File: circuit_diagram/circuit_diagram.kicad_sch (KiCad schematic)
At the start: 26 parts, among them J1 Sheild Power, M1 Stepper_Motor_bipolar, M2 Stepper_Motor_bipolar, M3 Stepper_Motor_bipolar, M4 Stepper_Motor_bipolar, M5 Motor_DC, SW1 SW_DPST_x2, SW2 SW_Push, U1 DEVKIT_V1_ESP32-WROOM-32

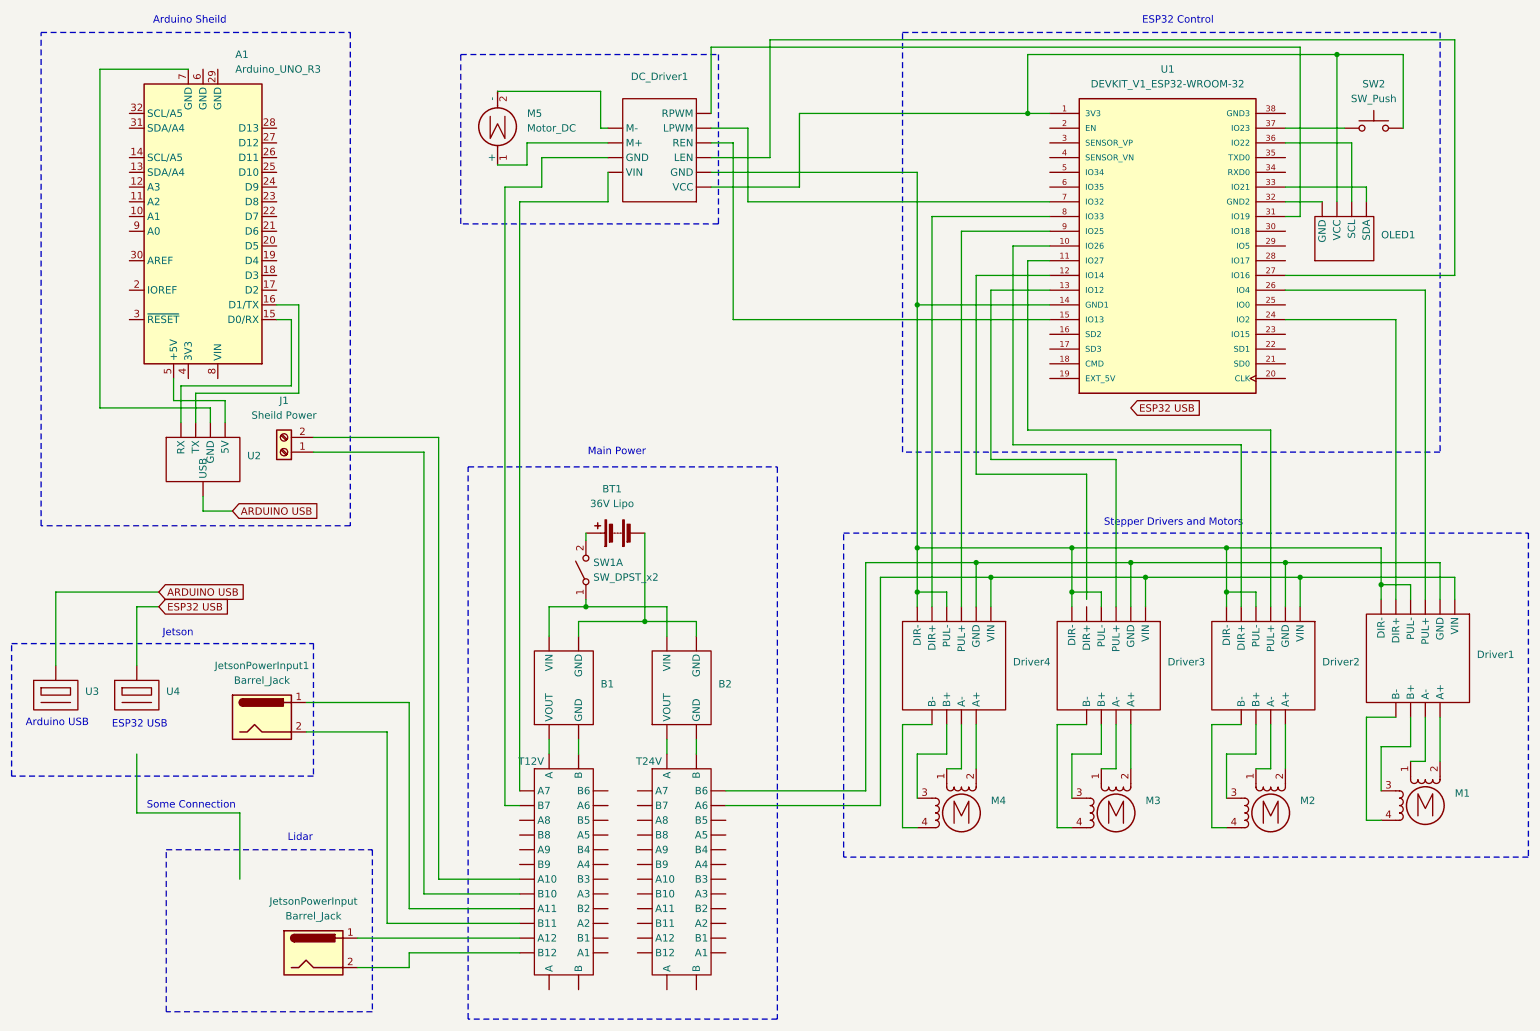
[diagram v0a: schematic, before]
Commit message: Drill Driver
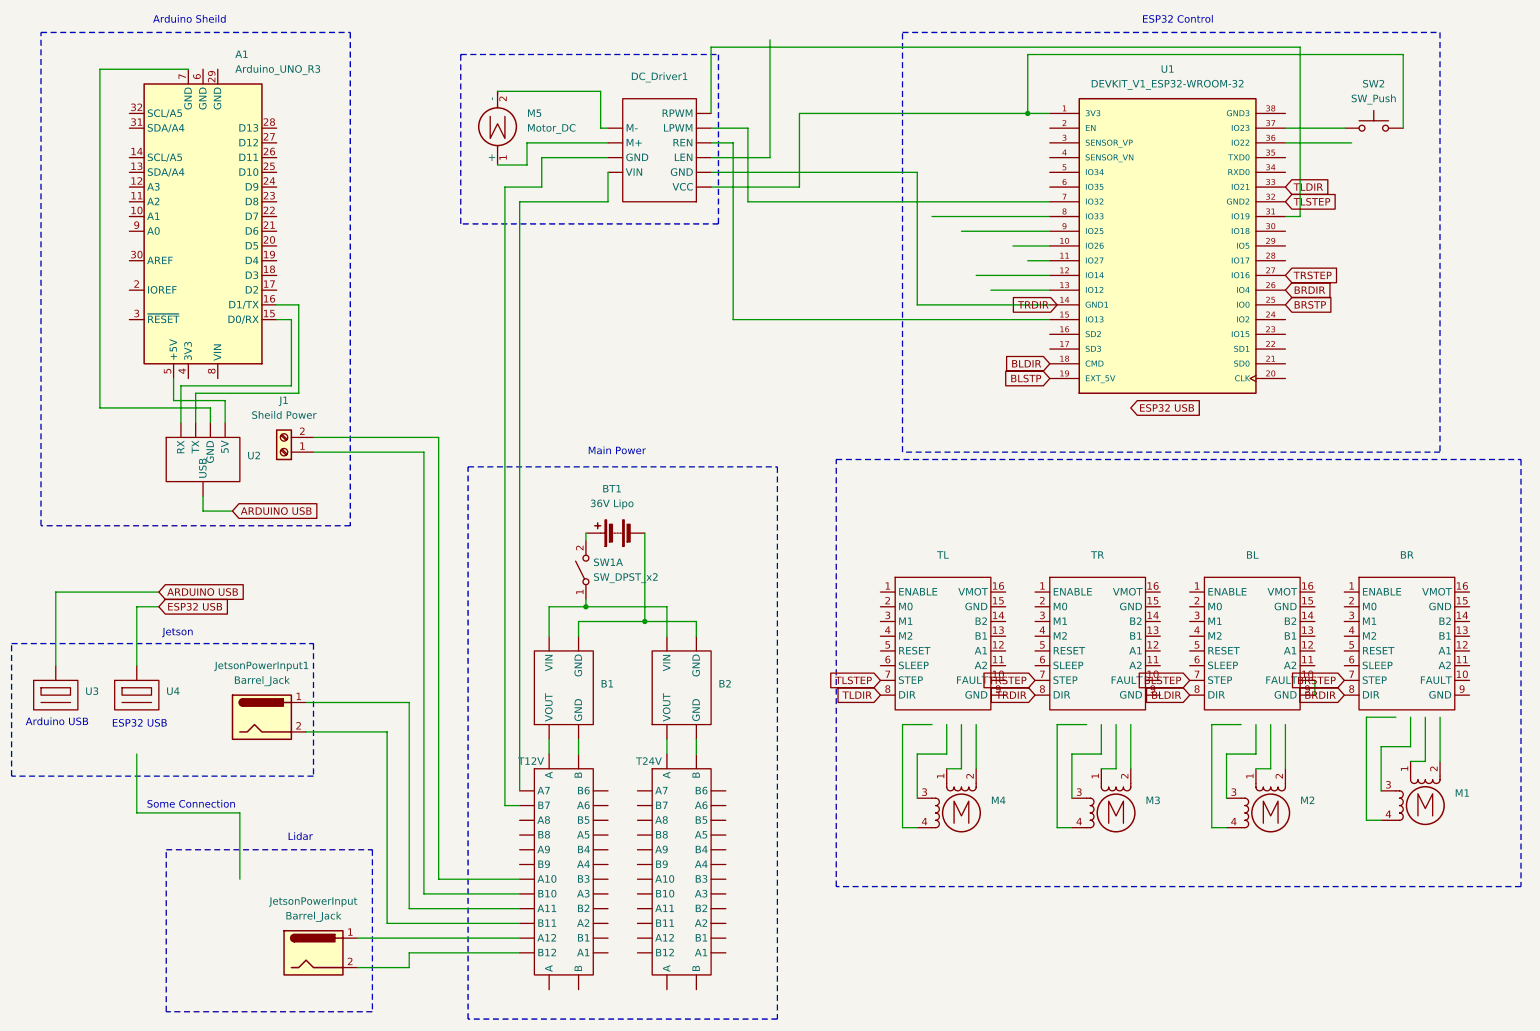
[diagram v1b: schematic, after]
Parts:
- removed Driver1, Driver2, Driver3, Driver4: ~, symbol components:Stepper Driver
- removed OLED1: ~, symbol components:OLED_SSD1306
- added BL, BR, TL, TR: ~, symbol components:DRV8825
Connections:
- net at B1. (VOUT): now also B2. (VOUT), SW1.1 (A); no longer T12V. (B9)
- net at T12V. (B9): now also J1.2 (Pin_2); no longer B1. (VOUT)
- net at DC_Driver1. (VIN): now also U1.7 (IO32); no longer T12V. (B9)
- net TRSTEP: now reaches U1.27 (IO16)
- net TRSTEP: now also TR.7 (STEP); no longer DC_Driver1. (VIN)
- net TLSTEP: now reaches U1.32 (GND2)
- net TLSTEP: now also TL.7 (STEP)
- net TLDIR: now reaches U1.33 (IO21)
- net TLDIR: now also TL.8 (DIR)
- net BRDIR: now reaches U1.26 (IO4)
- net BRDIR: now also BR.8 (DIR)
- net BLDIR: now reaches U1.18 (CMD)
- net BLDIR: now also BL.8 (DIR)
- net BLSTP: now reaches U1.19 (EXT_5V)
- net BRSTP: now reaches U1.25 (IO0)
- new net: B1. (VOUT), T12V. (B9) (x2)
- new net: B1. (VOUT), B2. (VOUT), BT1.2 (-)
- new net: DC_Driver1. (VIN), T12V. (B9) (x2)
- new net: B2. (VOUT), T24V. (B9)
- new net: BL.10 (FAULT), BL.9 (GND)
- new net BLSTEP: BL.7 (STEP)
- new net BRSTEP: BR.7 (STEP)
- new net TRDIR: TR.8 (DIR)
- now unconnected: T24V. (B9), T24V. (B9)
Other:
- note removed: "Stepper Drivers and Motors"
